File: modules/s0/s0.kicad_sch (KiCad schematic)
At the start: 0 parts

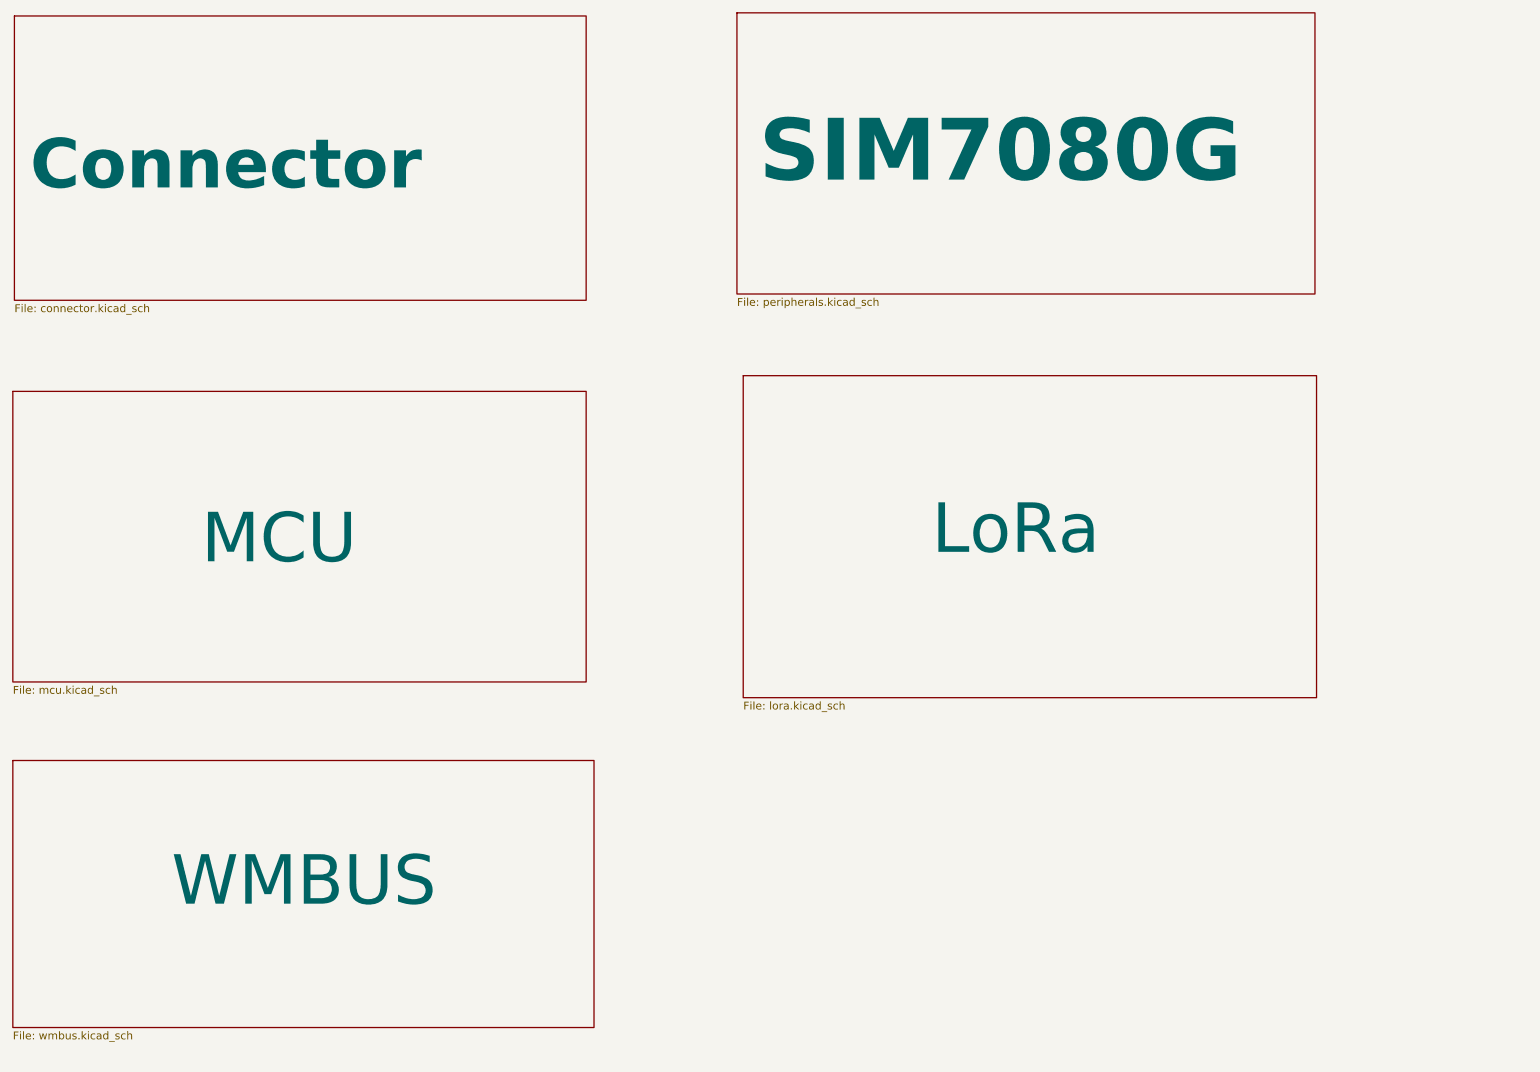
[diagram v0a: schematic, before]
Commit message: chore: add production files
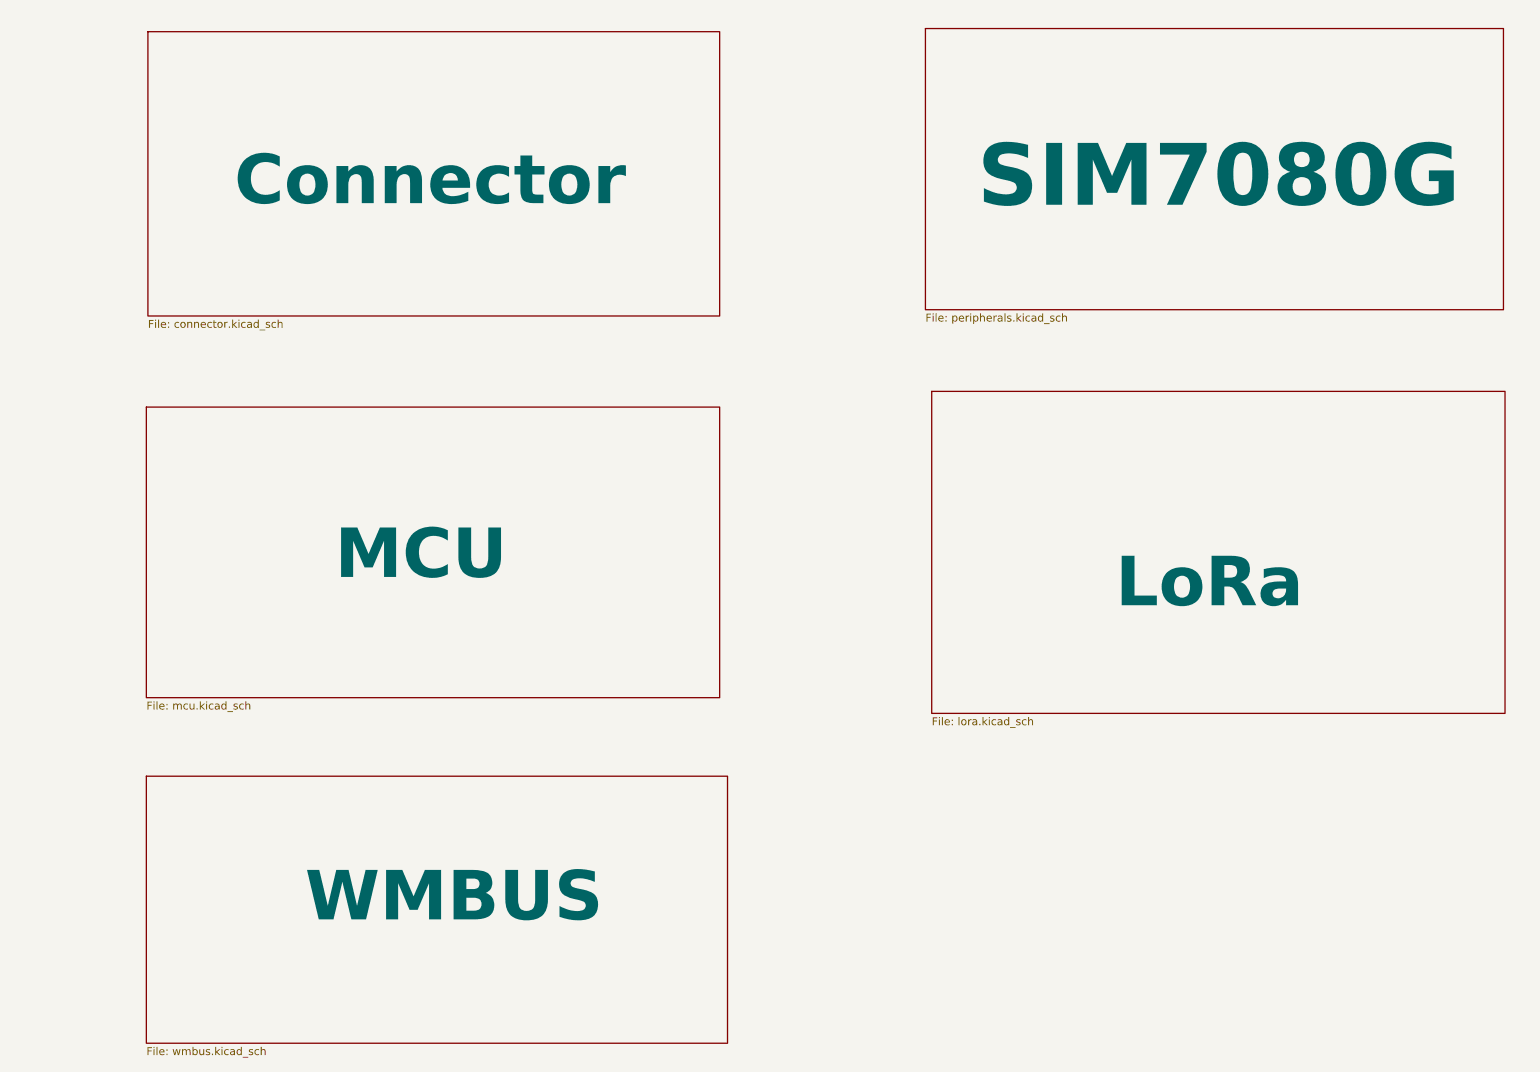
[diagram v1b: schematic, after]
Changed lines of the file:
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@@
 	)
 	(sheet
-		(at 21.59 138.43)
+		(at 43.18 140.97)
 		(size 93.98 43.18)
 		(stroke
@@
 		)
 		(property "Sheetname" "WMBUS"
-			(at 47.244 162.56 0)
+			(at 68.834 165.1 0)
 			(effects
 				(font
 					(size 8 8)
+					(thickness 1.6)
+					(bold yes)
 				)
 				(justify left bottom)
@@
 		)
 		(property "Sheetfile" "wmbus.kicad_sch"
-			(at 21.59 182.1946 0)
+			(at 43.18 184.7346 0)
 			(effects
 				(font
@@
 	)
 	(sheet
-		(at 21.59 78.74)
+		(at 43.18 81.28)
 		(size 92.71 46.99)
 		(stroke
@@
 		)
 		(property "Sheetname" "MCU"
-			(at 52.07 107.188 0)
+			(at 73.66 109.728 0)
 			(effects
 				(font
 					(size 8 8)
+					(thickness 1.6)
+					(bold yes)
 				)
 				(justify left bottom)
@@
 		)
 		(property "Sheetfile" "mcu.kicad_sch"
-			(at 21.59 126.3146 0)
+			(at 43.18 128.8546 0)
 			(effects
 				(font
@@
 	)
 	(sheet
-		(at 138.684 17.526)
+		(at 169.164 20.066)
 		(size 93.472 45.466)
 		(stroke
@@
 		)
 		(property "Sheetname" "SIM7080G"
-			(at 142.24 45.72 0)
+			(at 177.546 49.784 0)
 			(effects
 				(font
@@
 		)
 		(property "Sheetfile" "peripherals.kicad_sch"
-			(at 138.684 63.5766 0)
+			(at 169.164 66.1166 0)
 			(effects
 				(font
@@
 	)
 	(sheet
-		(at 21.844 18.034)
+		(at 43.434 20.574)
 		(size 92.456 45.974)
 		(stroke
@@
 		)
 		(property "Sheetname" "Connector"
-			(at 24.384 46.736 0)
+			(at 57.404 49.276 0)
 			(effects
 				(font
@@
 		)
 		(property "Sheetfile" "connector.kicad_sch"
-			(at 21.844 64.5926 0)
+			(at 43.434 67.1326 0)
 			(effects
 				(font
@@
 	)
 	(sheet
-		(at 139.7 76.2)
+		(at 170.18 78.74)
 		(size 92.71 52.07)
 		(stroke
@@
 		)
 		(property "Sheetname" "LoRa"
-			(at 170.18 105.664 0)
+			(at 199.898 114.3 0)
 			(effects
 				(font
 					(size 8 8)
+					(thickness 1.6)
+					(bold yes)
 				)
 				(justify left bottom)
@@
 		)
 		(property "Sheetfile" "lora.kicad_sch"
-			(at 139.7 128.8546 0)
+			(at 170.18 131.3946 0)
 			(effects
 				(font
